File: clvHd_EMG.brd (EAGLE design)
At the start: 21 x 18.5 mm, 25 parts, among them J1 XF2J-1824-12, J2 XF2J-1824-12, U1 ADS1293CISQ/NOPB

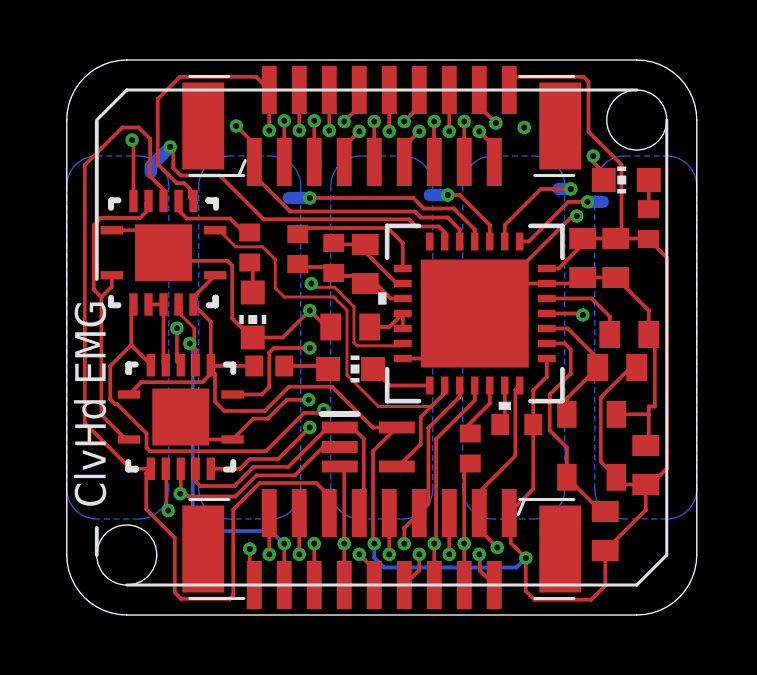
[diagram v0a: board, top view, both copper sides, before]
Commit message: shrinken
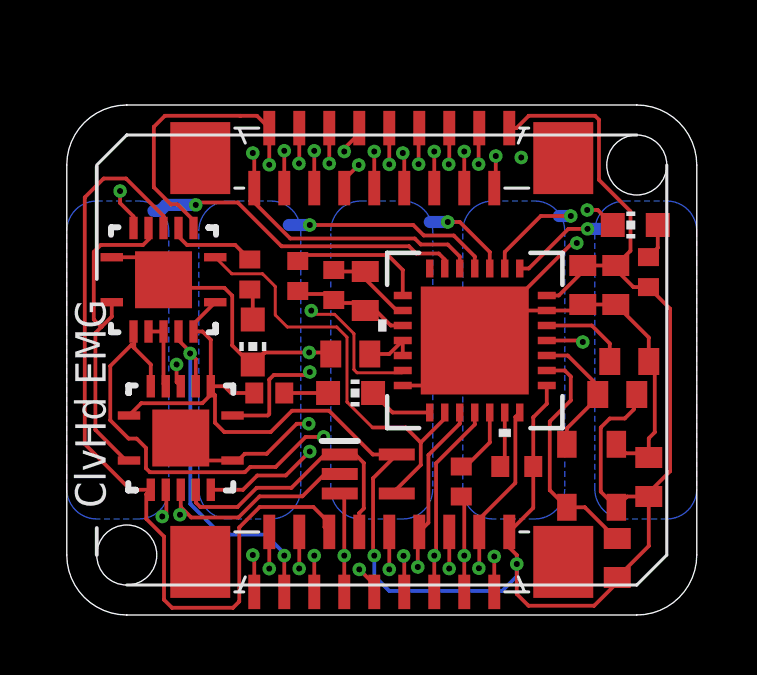
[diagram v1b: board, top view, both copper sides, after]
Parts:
- removed J1, J2: XF2J-1824-12, con-omron:XF2J-1824-12
- added 1, 2: X05C2018TZ, con-omron:X05C2018TZ
- moved R7 1.60 mm to (19.4, 11.4)
- moved L1 1.53 mm to (18.9, 13.0)
- moved R13 1.40 mm to (15.0, 4.95)
- moved R10 1.14 mm to (13.2, 4.45)
- moved U$1 1.00 mm to (17.5, 4.64)
- moved C10 0.98 mm to (18.4, 1.90)
- moved C12 0.90 mm to (9.45, 8.70)
- moved C16 0.90 mm to (17.2, 11.0)
- moved C19 0.90 mm to (18.3, 11.0)
- moved C20 0.90 mm to (18.8, 8.45)
- moved C9 0.90 mm to (18.4, 7.35)
- moved L3 0.90 mm to (6.20, 9.10)
- moved R1 0.90 mm to (6.10, 11.3)
- moved R12 0.90 mm to (6.75, 7.40)
- moved R15 0.90 mm to (8.90, 11.0)
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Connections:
- net A0: now also 1.3; no longer J1.16
- net A1: now also 1.5; no longer J1.14
- net A2: now also 1.6; no longer J1.13
- net A3: now also 1.8; no longer J1.11
- net CLK: now also 1.16, 2.3; no longer J1.3, J2.16
- net DIN: now also 1.13, 2.6; no longer J1.6, J2.13
- net DOUT: now also 1.15, 2.4; no longer J1.4, J2.15
- net GND: now also 1.11, 1.14, 1.17, 1.4, 1.7, 2.12, 2.15, 2.2, 2.5, 2.8; no longer J1.12, J1.15, J1.2, J1.5, J1.8, J2.11, J2.14, J2.17, J2.4, J2.7
- net GPIO1: now also 1.2, 2.17; no longer J1.17, J2.2
- net IN5: now also 1.1, 2.18; no longer J1.18, J2.1
- net RST: now also 1.9, 2.10; no longer J1.10, J2.9
- net S0: now also 2.16; no longer J2.3
- net S1: now also 2.14; no longer J2.5
- net S2: now also 2.13; no longer J2.6
- net S3: now also 2.11; no longer J2.8
- net SCLK: now also 1.12, 2.7; no longer J1.7, J2.12
- net SYNCB: now also 1.10, 2.9; no longer J1.9, J2.10
- net VDD: now also 1.18, 2.1; no longer J1.1, J2.18
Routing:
- net GND: track 54.7 -> 52.1 mm
- net A2: track 30.4 -> 27.8 mm
- net DOUT: track 19.6 -> 18.0 mm
- net N$16: track 21.5 -> 19.9 mm
- net S2: track 24.9 -> 23.5 mm
- net DIN: track 22.6 -> 21.3 mm
- net CLK: track 21.7 -> 20.5 mm
- net VDD: track 69.2 -> 68.0 mm
- net IN6: track 12.1 -> 10.9 mm
- net IN5: track 25.4 -> 24.3 mm
- net GPIO1: track 25.1 -> 24.1 mm
- net SYNCB: track 23.7 -> 22.8 mm
- net SCLK: track 21.4 -> 20.4 mm
- net A0: track 12.8 -> 12.2 mm
- net S3: track 17.0 -> 16.4 mm
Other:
- board size 21 x 18.5 mm -> 21 x 17 mm
- board text added: "ads1293-v2.2"
- board text removed: "ads1293-v2.1"
